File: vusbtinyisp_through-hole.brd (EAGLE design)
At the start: 36.2 x 20.3 mm, 9 parts, among them U1 Tiny85-20-SMT

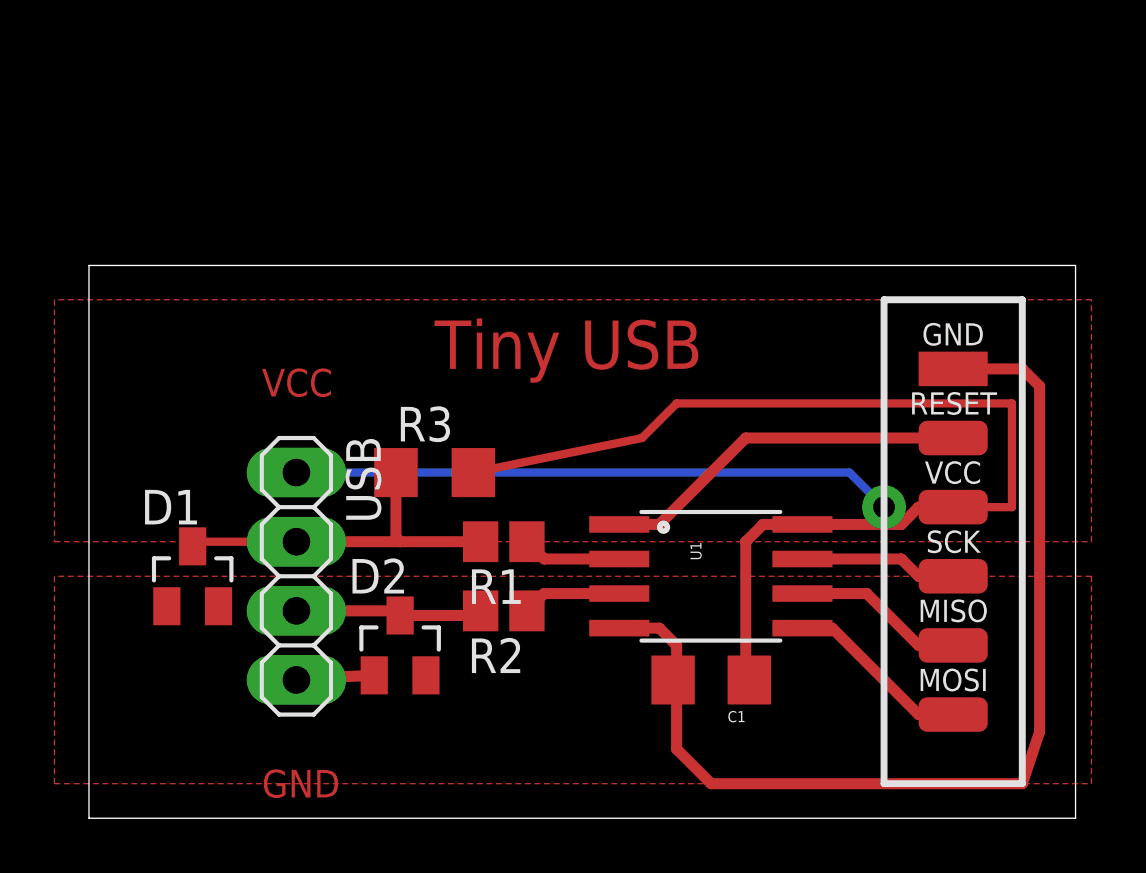
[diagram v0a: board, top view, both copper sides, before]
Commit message: complete, untested dip version
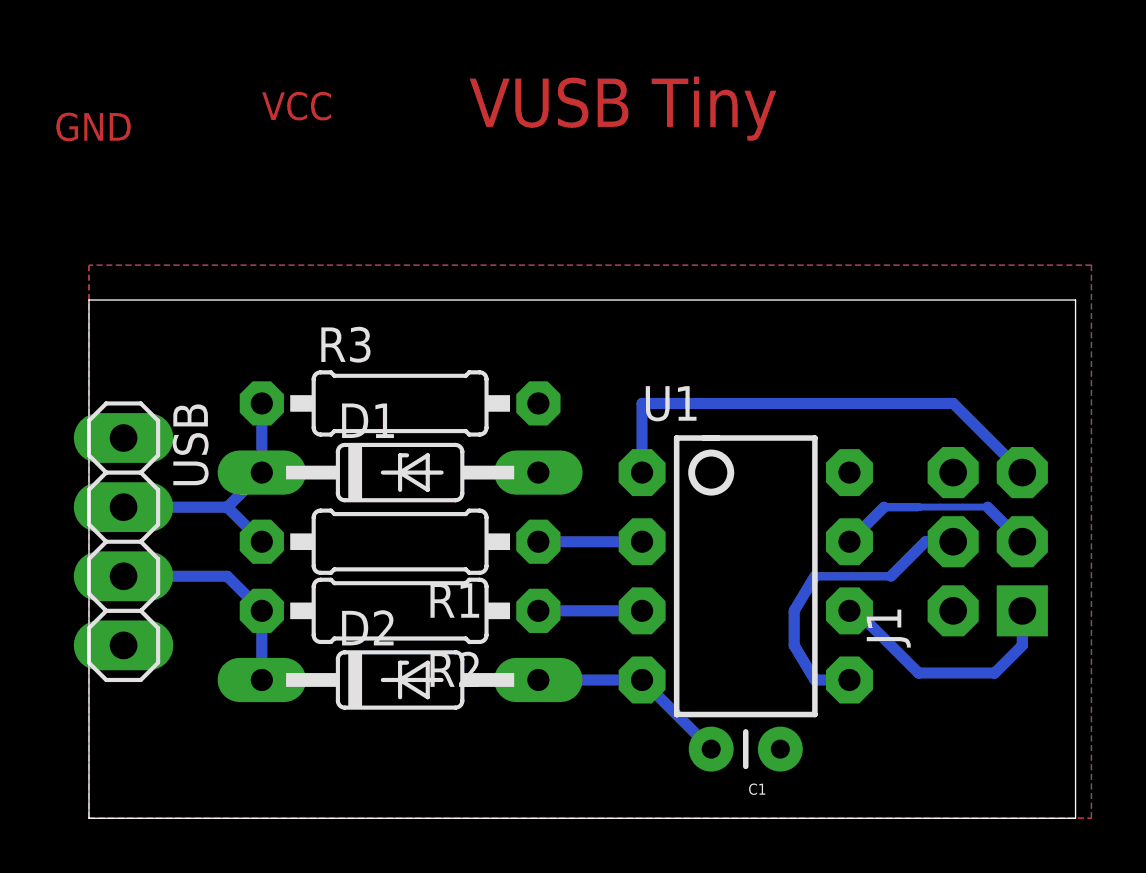
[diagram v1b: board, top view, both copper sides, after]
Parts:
- removed U$1: SMT_ISP, elliot:SMT_PADS
- added J1: AVR_SPI_PRG_6NS, SparkFun-Connectors:2X3-NS
- C1: device SparkFun-Passives:1206 -> SparkFun-Passives:CAP-PTH-SMALL
- D1, D2: device diode:SOT23 -> diode:DO35Z10
- R1, R2: device resistor:R0805 -> resistor:0207/10
- R3: device resistor:R1206 -> resistor:0207/10
- U1: value Tiny85-20-SMT -> TINY45-20-DIP; device SparkFun-DigitalIC:SO08-EIAJ -> SparkFun-DigitalIC:DIP08
- moved D1 8.52 mm to (40.6, 41.9)
- moved USB 6.48 mm to (30.5, 39.4)
- moved R1 3.81 mm to (40.6, 39.4)
- moved R2 3.81 mm to (40.6, 36.8)
- moved C1 3.59 mm to (54.6, 31.8)
- moved R3 2.84 mm to (40.6, 44.5)
- moved D2 1.27 mm to (40.6, 34.3)
- moved U1 1.27 mm to (53.3, 38.1)
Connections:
- net D+: now also D2.C; no longer D2.3
- net D-: now also D1.C; no longer D1.3
- net GND: now also D1.A, D2.A, J1.6; no longer D1.1, D2.1, U$1.GND
- net MISO: now also J1.1; no longer U$1.MISO
- net MOSI: now also J1.4; no longer U$1.MOSI
- net RESET: now also J1.5; no longer U$1.RST
- net SCK: now also J1.3; no longer U$1.SCK
- net VCC: now also J1.2; no longer U$1.VCC
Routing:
- net VCC: track 63.1 -> 0.00 mm, vias 1 -> 0
- net GND: track 42.8 -> 7.40 mm
- net MOSI: track 6.85 -> 11.1 mm
- net RESET: track 13.6 -> 17.6 mm
- net D-: track 13.4 -> 9.94 mm
- net MISO: track 6.33 -> 8.99 mm
- net SCK: track 5.80 -> 7.40 mm
- net D+: track 6.91 -> 8.15 mm
- added copper zone on layer 16, net GND
- removed copper zone on layer 1, net GND
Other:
- board size 36.2 x 20.3 mm -> 36.2 x 19 mm
- board text added: "VUSB Tiny"
- board text removed: "Tiny USB"

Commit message: changing 1k to 1.5k resistors in 5V designs
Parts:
- R3: value 1k Ohm -> 1.5k Ohm
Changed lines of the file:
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@@
 <element name="R1" library="resistor" package="0207/10" value="68ohm" x="40.64" y="39.37" rot="R180"/>
 <element name="R2" library="resistor" package="0207/10" value="68 ohm" x="40.64" y="36.83" rot="R180"/>
-<element name="R3" library="resistor" package="0207/10" value="1k Ohm" x="40.64" y="44.45"/>
+<element name="R3" library="resistor" package="0207/10" value="1.5k Ohm" x="40.64" y="44.45"/>
 <element name="J1" library="SparkFun-Connectors" package="2X3-NS" value="AVR_SPI_PRG_6NS" x="62.23" y="39.37" rot="R90"/>
 </elements>
